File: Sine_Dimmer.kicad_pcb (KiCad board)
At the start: 2 copper layers, 51 parts, among them J1 Input, J2 Output, Q1 IPW60R037P7, Q2 IPW60R037P7, Q3 IPW60R037P7, Q4 IPW60R037P7, U1 LT1711, U2 TLP2745, U3 TLP2745, U4 2EDN7424F, U5 UCC20520, U6 ESP-12E

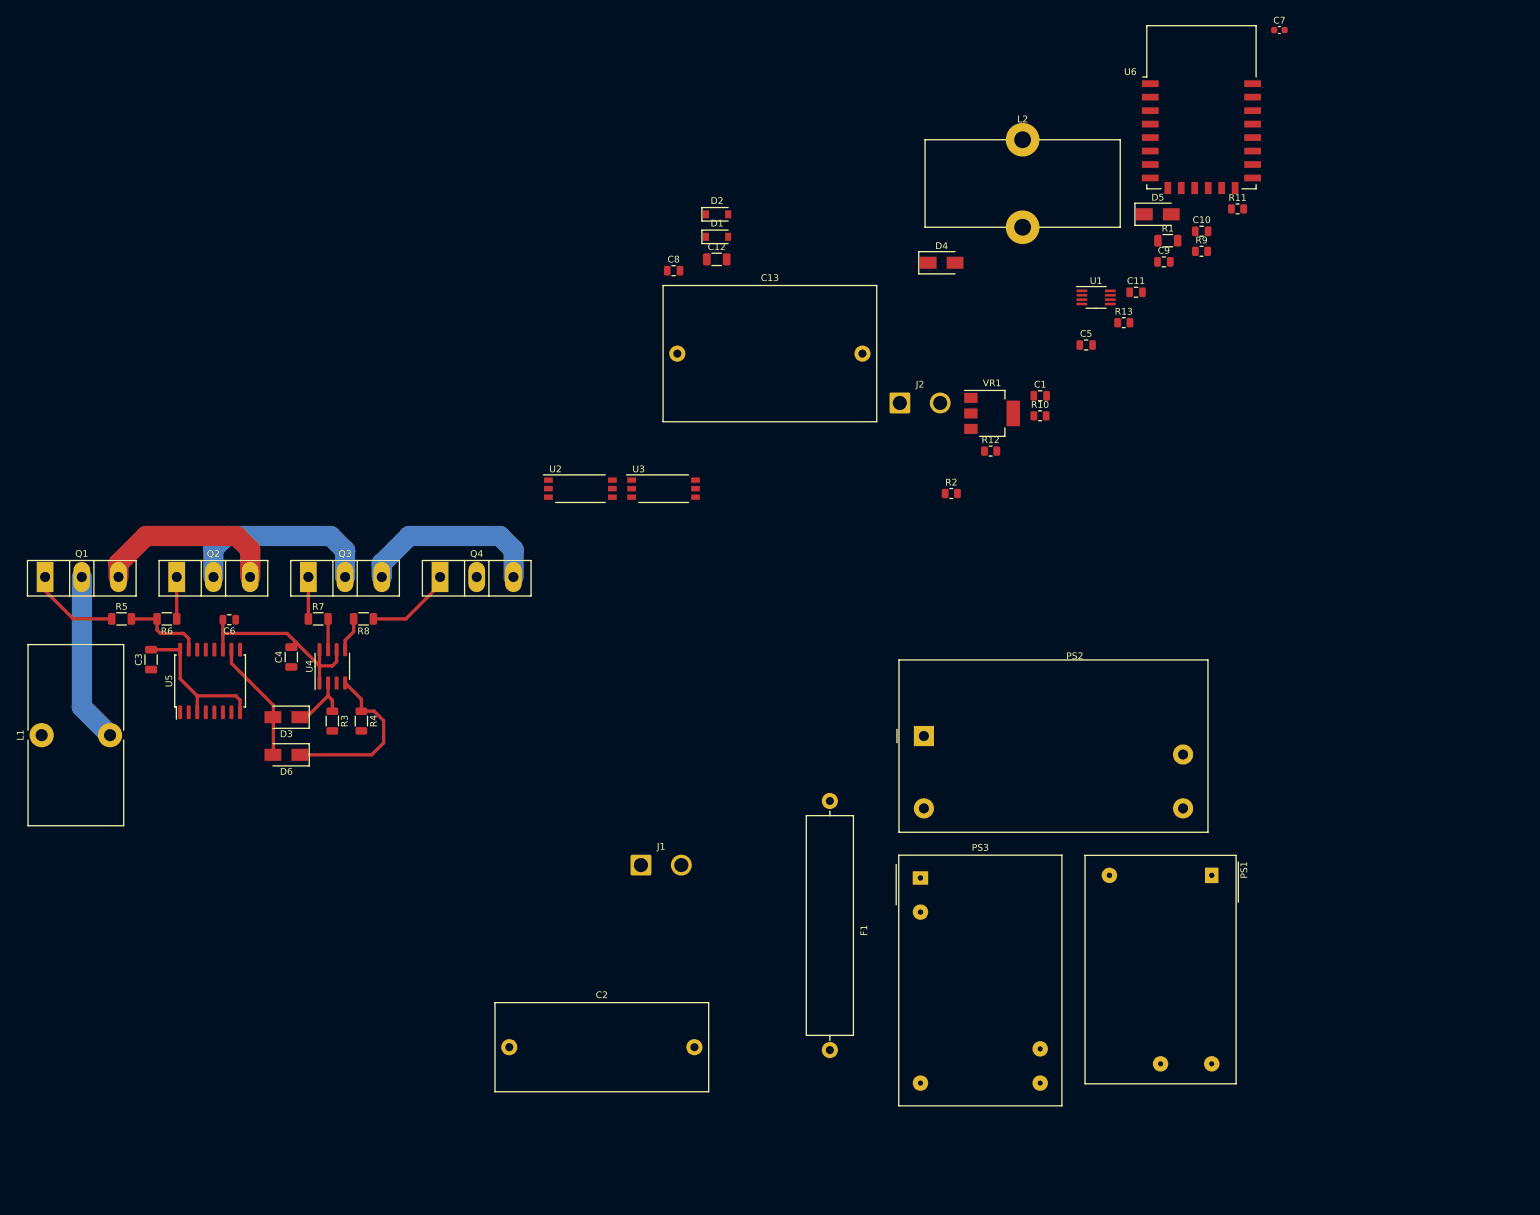
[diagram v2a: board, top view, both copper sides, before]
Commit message: Initial Release
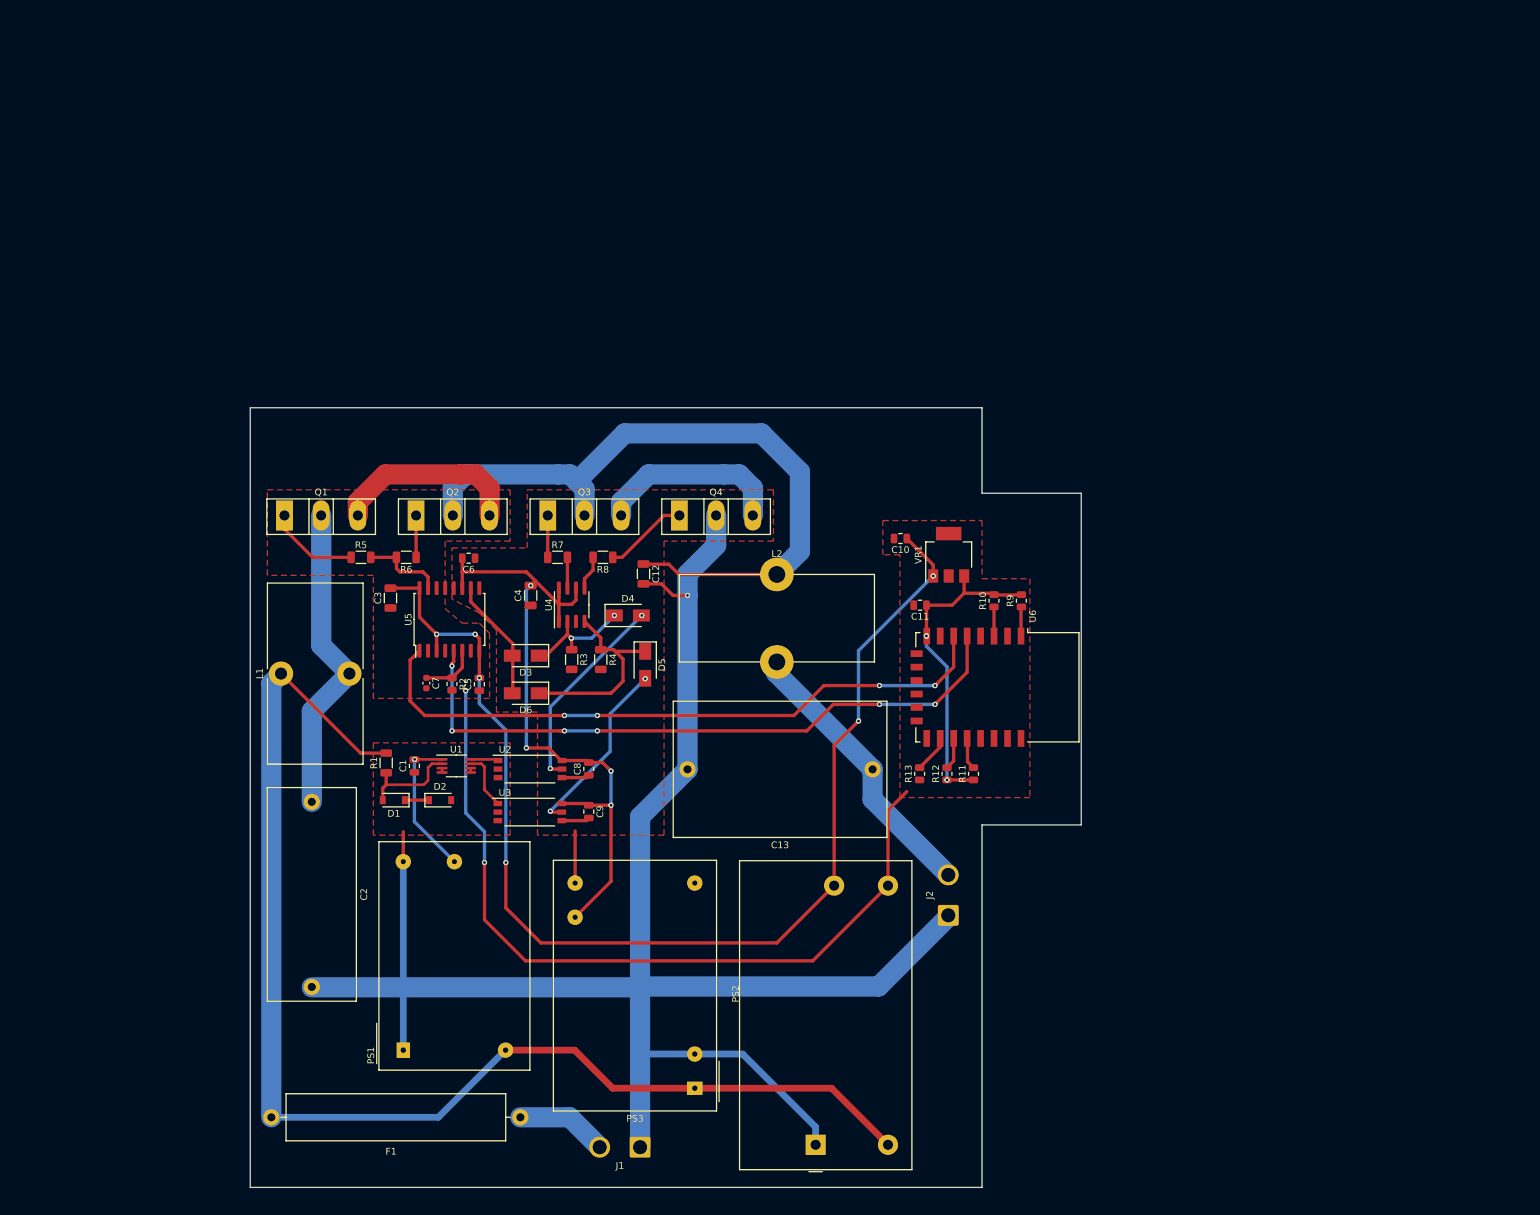
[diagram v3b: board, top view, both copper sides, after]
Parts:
- moved C7 159.6 mm to (114.6, 76.0), turned to 270 degrees
- moved R1 139.7 mm to (108.6, 87.8), turned to 90 degrees
- moved PS1 122.9 mm to (111.1, 130.5), turned to 90 degrees
- moved C9 118.2 mm to (138.7, 95.1), turned to 270 degrees
- moved U1 117.8 mm to (119.0, 88.3)
- moved C1 108.0 mm to (112.8, 88.3), turned to 90 degrees
- moved C5 103.3 mm to (122.4, 76.1), turned to 90 degrees
- moved D5 101.4 mm to (147.1, 73.2), turned to 270 degrees
- moved D1 96.5 mm to (109.7, 93.3), turned to 180 degrees
- moved D2 96.3 mm to (116.6, 93.3)
- moved R11 92.6 mm to (195.8, 89.4), turned to 90 degrees
- moved U6 91.3 mm to (199.4, 76.6), turned to 270 degrees
- moved F1 83.6 mm to (91.5, 140.5), turned to 0 degrees
- moved R2 79.4 mm to (118.4, 76.1), turned to 270 degrees
- moved J2 76.5 mm to (192.1, 110.5), turned to 90 degrees
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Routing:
- net NEUT: track 0.00 -> 272.0 mm, vias 0 -> 1
- net LINE: track 0.00 -> 188.6 mm
- net VCC: track 23.2 -> 176.8 mm, vias 0 -> 6
- net GND: track 28.2 -> 145.6 mm, vias 0 -> 2
- net dis: track 0.00 -> 97.5 mm, vias 0 -> 6
- net pwm: track 0.00 -> 97.2 mm, vias 0 -> 4
- net Net-(C12-Pad1): track 29.4 -> 104.9 mm
- net VDD: track 31.3 -> 101.0 mm, vias 0 -> 4
- net Net-(C11-Pad1): track 0.00 -> 48.7 mm, vias 0 -> 2
- net VPP: track 0.00 -> 42.2 mm
- net rev: track 0.00 -> 30.1 mm, vias 0 -> 2
- net fwd: track 0.00 -> 27.3 mm, vias 0 -> 2
- net Net-(C1-Pad2): track 0.00 -> 21.8 mm, vias 0 -> 1
- net Net-(C2-Pad1): track 25.2 -> 46.6 mm
- net VSS: track 28.2 -> 44.2 mm
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- added copper zone on F.Cu, net GND
- added copper zone on F.Cu, net NEUT
- added copper zone on F.Cu, net VSS
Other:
- board outline added: 123.4 x 115.8 mm
